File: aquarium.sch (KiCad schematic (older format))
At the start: 32 parts

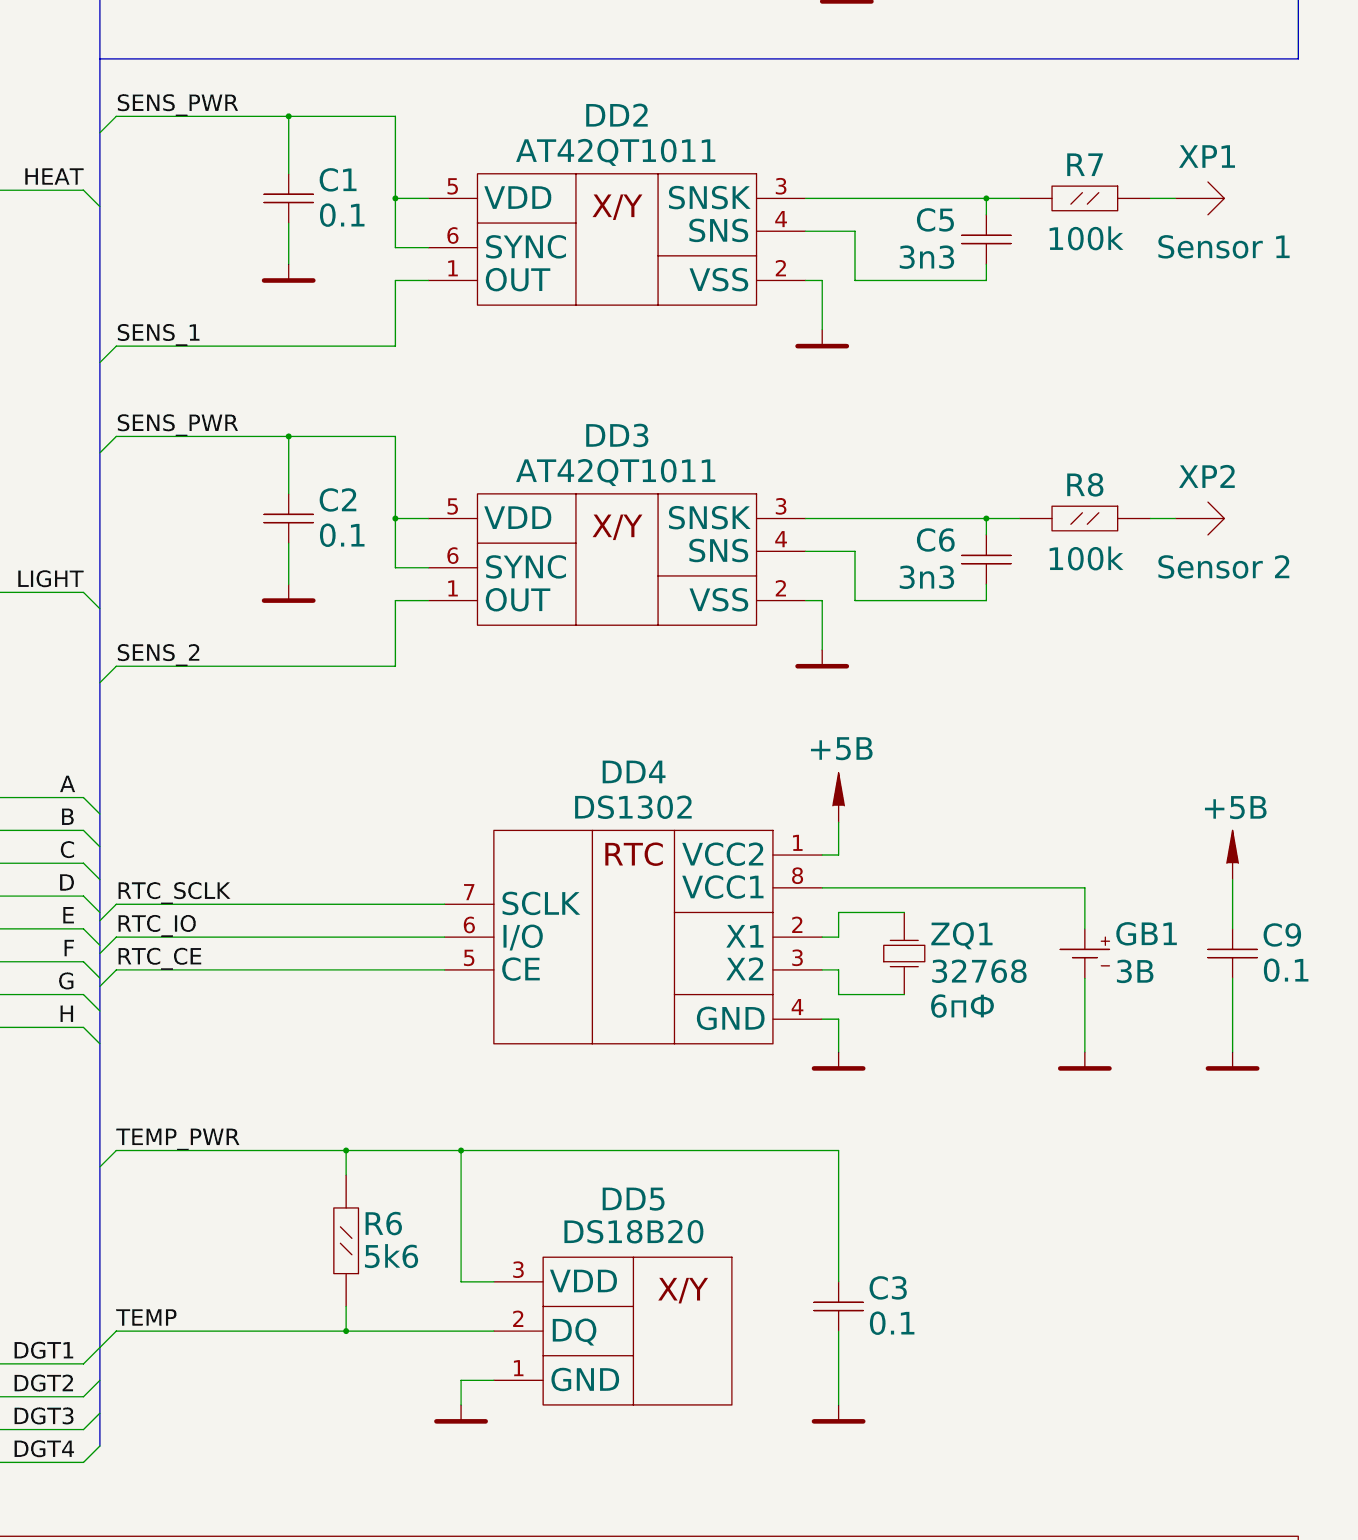
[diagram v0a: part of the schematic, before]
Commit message: New version of the schematic and PCB's.
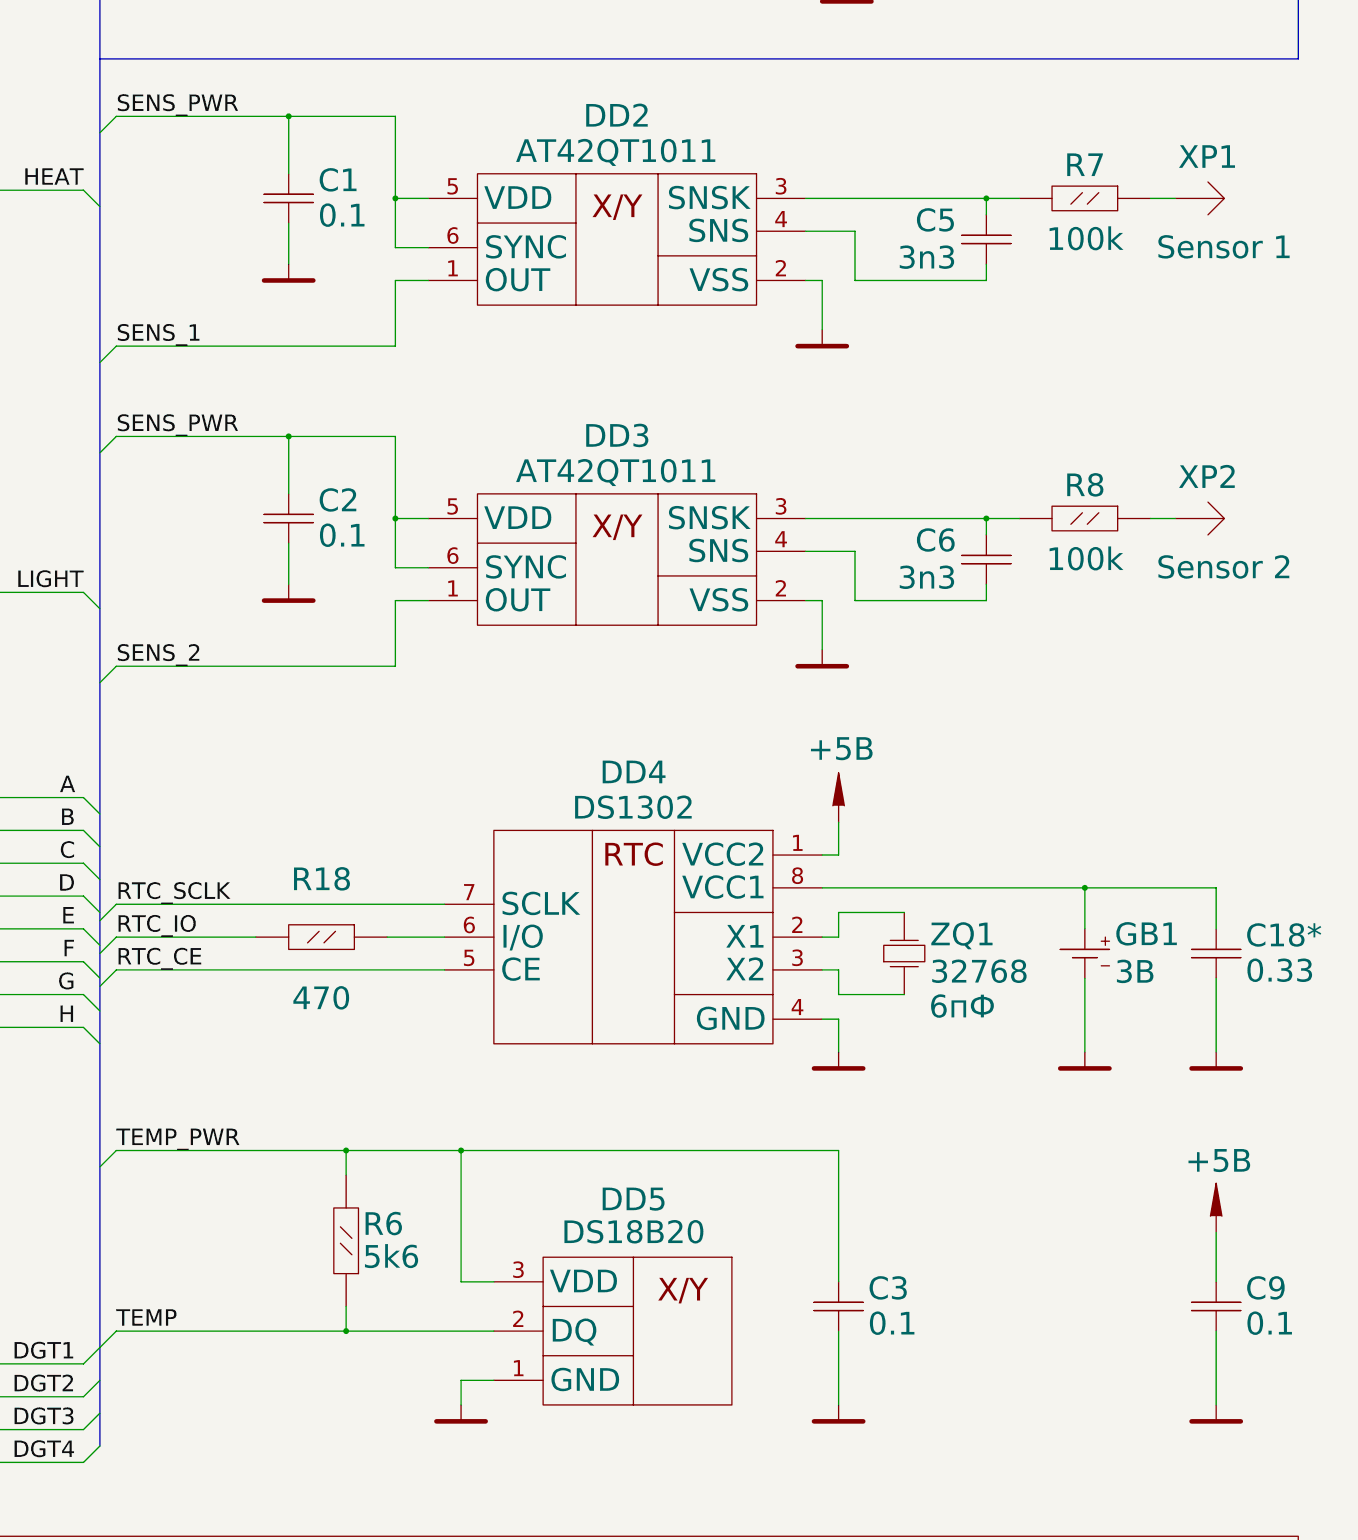
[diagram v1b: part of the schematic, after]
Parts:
- added C18*: 0.33, Конденсаторы:SMD_0805, symbol C
- added R18: 470, Резисторы:R_0805, symbol R.125
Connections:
- net GND: now also C18*.2
- net RTC_IO: now also R18.2; no longer DD4.6 (I/O)
- net at DD4.8 (VCC1), GB1.1 (+): now also C18*.1
- new net: DD4.6 (I/O), R18.1
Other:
- moved on the sheet: C9
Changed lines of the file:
@@
 $EndComp
 $Comp
-L GND #PWR01
+L GND #PWR17
 U 1 1 56791BEA
 P 9500 1550
-F 0 "#PWR01" H 9900 1550 138 0001 C CNN
+F 0 "#PWR17" H 9900 1550 138 0001 C CNN
 F 1 "GND" H 9150 1550 138 0001 C CNN
 F 2 "" H 9500 1550 60  0000 C CNN
@@
 $EndComp
 $Comp
-L GND #PWR02
+L GND #PWR19
 U 1 1 56791C0B
 P 10200 1550
-F 0 "#PWR02" H 10600 1550 138 0001 C CNN
+F 0 "#PWR19" H 10600 1550 138 0001 C CNN
 F 1 "GND" H 9850 1550 138 0001 C CNN
 F 2 "" H 10200 1550 60  0000 C CNN
@@
 $EndComp
 $Comp
-L +5B #PWR03
+L +5B #PWR16
 U 1 1 56791C40
 P 9500 750
-F 0 "#PWR03" H 10000 850 138 0001 C CNN
+F 0 "#PWR16" H 10000 850 138 0001 C CNN
 F 1 "+5B" H 9484 1185 138 0000 C CNN
 F 2 "" H 9500 950 60  0000 C CNN
@@
 $EndComp
 $Comp
-L +5B #PWR04
+L +5B #PWR18
 U 1 1 56791C61
 P 10200 750
-F 0 "#PWR04" H 10700 850 138 0001 C CNN
+F 0 "#PWR18" H 10700 850 138 0001 C CNN
 F 1 "+5B" H 10184 1185 138 0000 C CNN
 F 2 "" H 10200 950 60  0000 C CNN
@@
 	10200 1300 10200 1550
 $Comp
-L +5B #PWR05
+L +5B #PWR14
 U 1 1 56791F4C
 P 8750 750
-F 0 "#PWR05" H 9250 850 138 0001 C CNN
+F 0 "#PWR14" H 9250 850 138 0001 C CNN
 F 1 "+5B" H 8734 1185 138 0000 C CNN
 F 2 "" H 8750 950 60  0000 C CNN
@@
 Connection ~ 8750 950
 $Comp
-L GND #PWR06
+L GND #PWR15
 U 1 1 567920EA
 P 8750 4550
-F 0 "#PWR06" H 9150 4550 138 0001 C CNN
+F 0 "#PWR15" H 9150 4550 138 0001 C CNN
 F 1 "GND" H 8400 4550 138 0001 C CNN
 F 2 "" H 8750 4550 60  0000 C CNN
@@
 $EndComp
 $Comp
-L GND #PWR07
+L GND #PWR6
 U 1 1 56795326
 P 5350 6250
-F 0 "#PWR07" H 5750 6250 138 0001 C CNN
+F 0 "#PWR6" H 5750 6250 138 0001 C CNN
 F 1 "GND" H 5000 6250 138 0001 C CNN
 F 2 "" H 5350 6250 60  0000 C CNN
@@
 L C C9
 U 1 1 5679539A
-P 11100 10450
-F 0 "C9" H 11278 10558 138 0000 L CNN
-F 1 "0.1" H 11278 10343 138 0000 L CNN
-F 2 "Конденсаторы:SMD_0805" H 11100 10475 60  0001 C CNN
-F 3 "" H 11100 10475 60  0000 C CNN
-	1    11100 10450
-	1    0    0    -1
-$EndComp
-$Comp
-L GND #PWR08
+P 11000 12600
+F 0 "C9" H 11178 12708 138 0000 L CNN
+F 1 "0.1" H 11178 12493 138 0000 L CNN
+F 2 "Конденсаторы:SMD_0805" H 11000 12625 60  0001 C CNN
+F 3 "" H 11000 12625 60  0000 C CNN
+	1    11000 12600
+	1    0    0    -1
+$EndComp
+$Comp
+L GND #PWR24
 U 1 1 567953A0
-P 11100 11050
-F 0 "#PWR08" H 11500 11050 138 0001 C CNN
-F 1 "GND" H 10750 11050 138 0001 C CNN
-F 2 "" H 11100 11050 60  0000 C CNN
-F 3 "" H 11100 11050 60  0000 C CNN
-	1    11100 11050
-	-1   0    0    -1
-$EndComp
-$Comp
-L +5B #PWR09
+P 11000 13200
+F 0 "#PWR24" H 11400 13200 138 0001 C CNN
+F 1 "GND" H 10650 13200 138 0001 C CNN
+F 2 "" H 11000 13200 60  0000 C CNN
+F 3 "" H 11000 13200 60  0000 C CNN
+	1    11000 13200
+	-1   0    0    -1
+$EndComp
+$Comp
+L +5B #PWR23
 U 1 1 567953A6
-P 11100 10000
-F 0 "#PWR09" H 11600 10100 138 0001 C CNN
-F 1 "+5B" H 11084 10435 138 0000 C CNN
-F 2 "" H 11100 10200 60  0000 C CNN
-F 3 "" H 11100 10200 60  0000 C CNN
-	1    11100 10000
-	-1   0    0    -1
-$EndComp
-Wire Wire Line
-	11100 10000 11100 10300
-Wire Wire Line
-	11100 10600 11100 11050
+P 11000 12150
+F 0 "#PWR23" H 11500 12250 138 0001 C CNN
+F 1 "+5B" H 10984 12585 138 0000 C CNN
+F 2 "" H 11000 12350 60  0000 C CNN
+F 3 "" H 11000 12350 60  0000 C CNN
+	1    11000 12150
+	-1   0    0    -1
+$EndComp
+Wire Wire Line
+	11000 12150 11000 12450
+Wire Wire Line
+	11000 12750 11000 13200
 $Comp
 L QUARTZ ZQ1
@@
 	8700 10200 9100 10200
 $Comp
-L +5B #PWR010
+L +5B #PWR11
 U 1 1 56797DB1
 P 8700 9650
-F 0 "#PWR010" H 9200 9750 138 0001 C CNN
+F 0 "#PWR11" H 9200 9750 138 0001 C CNN
 F 1 "+5B" H 8684 10094 138 0000 C CNN
 F 2 "" H 8700 9850 60  0000 C CNN
@@
 	8700 9850 8600 9850
 Wire Wire Line
-	8600 10050 10200 10050
+	8600 10050 11000 10050
 $Comp
 L C C5
@@
 $EndComp
 $Comp
-L GND #PWR011
+L GND #PWR12
 U 1 1 5679847B
 P 8700 11050
-F 0 "#PWR011" H 9100 11050 138 0001 C CNN
+F 0 "#PWR12" H 9100 11050 138 0001 C CNN
 F 1 "GND" H 8350 11050 138 0001 C CNN
 F 2 "" H 8700 11050 60  0000 C CNN
@@
 	9600 6350 9600 6250
 $Comp
-L GND #PWR012
+L GND #PWR9
 U 1 1 56798CBF
 P 8600 6650
-F 0 "#PWR012" H 9000 6650 138 0001 C CNN
+F 0 "#PWR9" H 9000 6650 138 0001 C CNN
 F 1 "GND" H 8250 6650 138 0001 C CNN
 F 2 "" H 8600 6650 60  0000 C CNN
@@
 $EndComp
 $Comp
-L GND #PWR013
+L GND #PWR8
 U 1 1 567A531F
 P 6400 13200
-F 0 "#PWR013" H 6800 13200 138 0001 C CNN
+F 0 "#PWR8" H 6800 13200 138 0001 C CNN
 F 1 "GND" H 6050 13200 138 0001 C CNN
 F 2 "" H 6400 13200 60  0000 C CNN
@@
 GND
 $Comp
-L GND #PWR014
+L GND #PWR2
 U 1 1 567D101C
 P 2000 6100
-F 0 "#PWR014" H 2400 6100 138 0001 C CNN
+F 0 "#PWR2" H 2400 6100 138 0001 C CNN
 F 1 "GND" H 1650 6100 138 0001 C CNN
 F 2 "" H 2000 6100 60  0000 C CNN
@@
 	6300 10150 4300 10150
 Wire Wire Line
-	6300 10350 4300 10350
+	6300 10350 5950 10350
+Wire Wire Line
+	4300 10350 5150 10350
 Entry Wire Line
 	4300 10550 4200 10650
@@
 $EndSheet
 $Comp
-L GND #PWR015
+L GND #PWR20
 U 1 1 58491DD9
 P 10200 11050
-F 0 "#PWR015" H 10600 11050 138 0001 C CNN
+F 0 "#PWR20" H 10600 11050 138 0001 C CNN
 F 1 "GND" H 9850 11050 138 0001 C CNN
 F 2 "" H 10200 11050 60  0000 C CNN
@@
 	2000 11800 2000 11950
 $Comp
-L +5B #PWR016
+L +5B #PWR4
 U 1 1 584B914C
 P 2650 4900
-F 0 "#PWR016" H 3150 5000 138 0001 C CNN
+F 0 "#PWR4" H 3150 5000 138 0001 C CNN
 F 1 "+5B" H 2634 5335 138 0000 C CNN
 F 2 "" H 2650 5100 60  0000 C CNN
@@
 $EndComp
 $Comp
-L GND #PWR017
+L GND #PWR13
 U 1 1 584EFF17
 P 8700 13200
-F 0 "#PWR017" H 9100 13200 138 0001 C CNN
+F 0 "#PWR13" H 9100 13200 138 0001 C CNN
 F 1 "GND" H 8350 13200 138 0001 C CNN
 F 2 "" H 8700 13200 60  0000 C CNN
@@
 Connection ~ 6400 11650
 $Comp
-L +12B #PWR018
+L +12B #PWR1
 U 1 1 58470EC2
 P 2000 4900
-F 0 "#PWR018" H 2500 5000 138 0001 C CNN
+F 0 "#PWR1" H 2500 5000 138 0001 C CNN
 F 1 "+12B" H 1987 5345 138 0000 C CNN
 F 2 "" H 2000 5100 60  0000 C CNN
@@
 	2000 4900 2000 5200
 $Comp
-L +12B #PWR019
+L +12B #PWR5
 U 1 1 586A2E7C
 P 2650 6900
-F 0 "#PWR019" H 3150 7000 138 0001 C CNN
+F 0 "#PWR5" H 3150 7000 138 0001 C CNN
 F 1 "+12B" H 2637 7345 138 0000 C CNN
 F 2 "" H 2650 7100 60  0000 C CNN
@@
 	2000 7400 2000 7700
 $Comp
-L GND #PWR020
+L GND #PWR3
 U 1 1 586A3FC9
 P 2000 8700
-F 0 "#PWR020" H 2400 8700 138 0001 C CNN
+F 0 "#PWR3" H 2400 8700 138 0001 C CNN
 F 1 "GND" H 1650 8700 138 0001 C CNN
 F 2 "" H 2000 8700 60  0000 C CNN
@@
 TEMP_PWR
 Wire Wire Line
-	6000 5350 4300 5350
+	4300 5350 6000 5350
 Entry Wire Line
 	4300 5350 4200 5450
@@
 $EndComp
 $Comp
-L GND #PWR021
+L GND #PWR7
 U 1 1 586F73E8
 P 5350 8200
-F 0 "#PWR021" H 5750 8200 138 0001 C CNN
+F 0 "#PWR7" H 5750 8200 138 0001 C CNN
 F 1 "GND" H 5000 8200 138 0001 C CNN
 F 2 "" H 5350 8200 60  0000 C CNN
@@
 	9600 8300 9600 8200
 $Comp
-L GND #PWR022
+L GND #PWR10
 U 1 1 586F7403
 P 8600 8600
-F 0 "#PWR022" H 9000 8600 138 0001 C CNN
+F 0 "#PWR10" H 9000 8600 138 0001 C CNN
 F 1 "GND" H 8250 8600 138 0001 C CNN
 F 2 "" H 8600 8600 60  0000 C CNN
@@
 SENS_2
 Wire Wire Line
-	6000 7300 4300 7300
+	4300 7300 6000 7300
 Entry Wire Line
 	4300 7300 4200 7400
@@
 $EndComp
 $Comp
-L GND #PWR023
+L GND #PWR21
 U 1 1 586F79F4
 P 10800 1550
-F 0 "#PWR023" H 11200 1550 138 0001 C CNN
+F 0 "#PWR21" H 11200 1550 138 0001 C CNN
 F 1 "GND" H 10450 1550 138 0001 C CNN
 F 2 "" H 10800 1550 60  0000 C CNN
@@
 Connection ~ 5350 5350
 Connection ~ 5350 7300
+$Comp
+L R.125 R18
+U 1 1 58978D6E
+P 5550 10350
+F 0 "R18" H 5550 10700 138 0000 C CNN
+F 1 "470" H 5550 9975 138 0000 C CNN
+F 2 "Резисторы:R_0805" H 5550 10350 60  0001 C CNN
+F 3 "" H 5550 10350 60  0000 C CNN
+	1    5550 10350
+	-1   0    0    -1
+$EndComp
+$Comp
+L C C18*
+U 1 1 58C4168F
+P 11000 10450
+F 0 "C18*" H 11178 10558 138 0000 L CNN
+F 1 "0.33" H 11178 10343 138 0000 L CNN
+F 2 "Конденсаторы:SMD_0805" H 11000 10475 60  0001 C CNN
+F 3 "" H 11000 10475 60  0000 C CNN
+	1    11000 10450
+	1    0    0    -1
+$EndComp
+$Comp
+L GND #PWR22
+U 1 1 58C41695
+P 11000 11050
+F 0 "#PWR22" H 11400 11050 138 0001 C CNN
+F 1 "GND" H 10650 11050 138 0001 C CNN
+F 2 "" H 11000 11050 60  0000 C CNN
+F 3 "" H 11000 11050 60  0000 C CNN
+	1    11000 11050
+	-1   0    0    -1
+$EndComp
+Wire Wire Line
+	11000 10050 11000 10300
+Wire Wire Line
+	11000 10600 11000 11050
+Connection ~ 10200 10050
 $EndSCHEMATC
